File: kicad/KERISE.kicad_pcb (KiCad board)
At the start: 2 copper layers, 46.5 x 50 mm, 145 parts, among them J1 COM, P1 ANT, P10 Partition, P11 PR_Host, P12 PR_Slave, P13 Partition, P14 Partition, P15 Partition, P16 Partition, P17 Fan, P18 ENC_Host, P19 ENC_Slave, P2 Motor_L, P20 ToF_Host, P21 ToF_Slave, P22 ENC_Host, P23 ENC_Slave, P24 PR_Host, P25 PR_Slave, P26 Partition, P27 Partition, P28 Partition, P29 Partition, P3 Motor_R, P30 PR_Host, P31 PR_Slave, P32 Partition, P33 Partition, P34 Partition, P35 Partition, P4 Battery, P5 PR_Host, P6 PR_Slave, P7 Partition, P8 Partition, P9 Partition, Q1 DMN3065LW-7, Q2 DMN3065LW-7, Q3 NX3020NAKW, Q4 DMN3065LW-7, Q5 DMN3065LW-7, Q6 DMN3065LW-7, SW1 SW_Push, SW2 SW_Push, U1 FLASH, U10 AS5048A, U11 ICM-20602, U12 AD8601, U13 AD8601, U2 ESP32, U3 XTAL, U4 DRV8835, U5 LXDC2URxx, U6 AD8601, U7 AD8601, U8 AS5048A, U9 VL53L0X

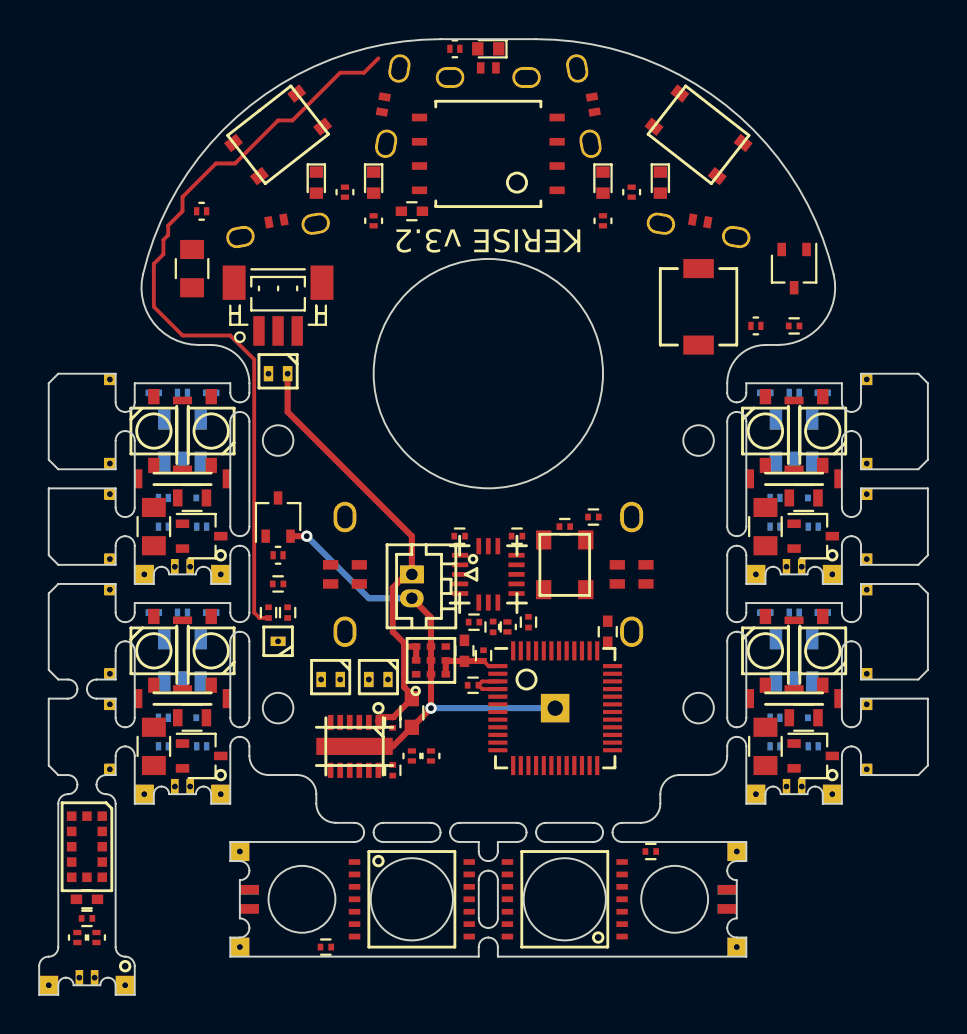
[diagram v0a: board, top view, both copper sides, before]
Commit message: 配線完了
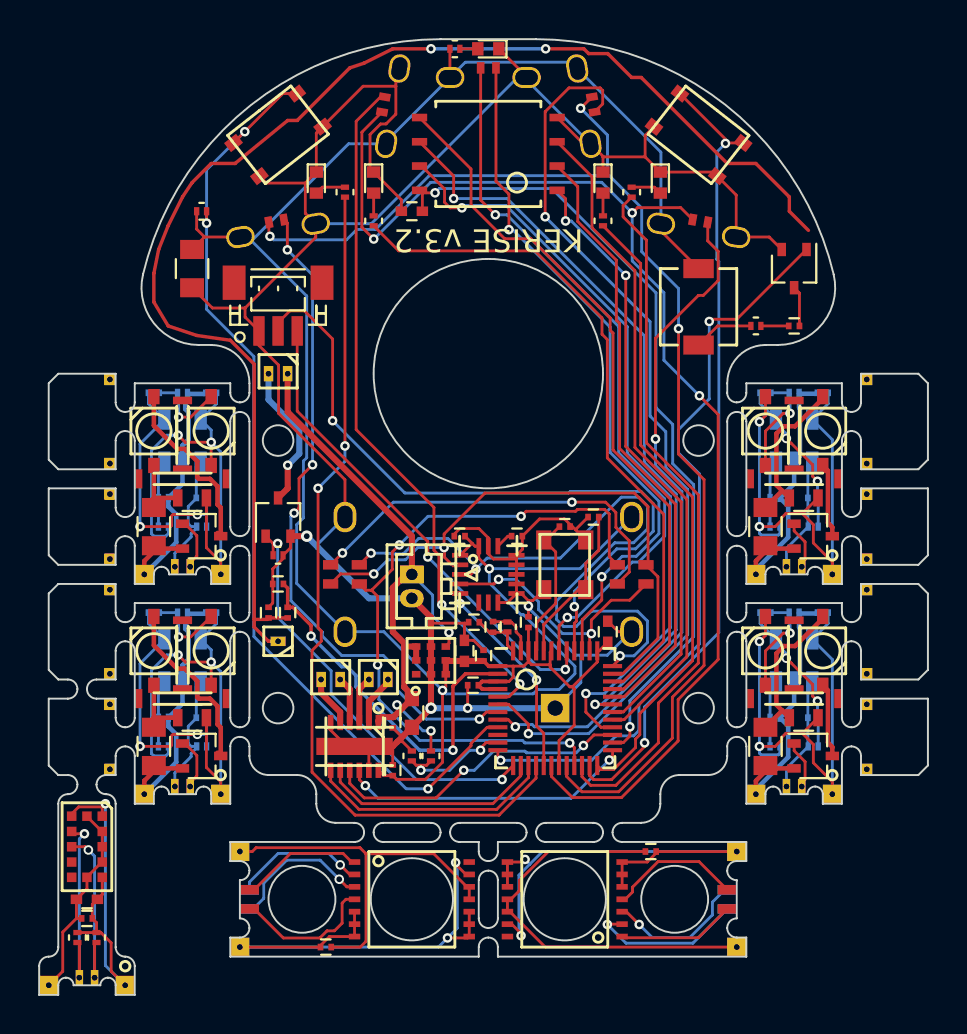
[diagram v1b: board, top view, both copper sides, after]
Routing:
- net GND: track 25.2 -> 155.0 mm, vias 2 -> 4
- net +3V3: track 6.01 -> 127.3 mm, vias 0 -> 2
- net PR-LED-SL: track 0.00 -> 65.5 mm, vias 0 -> 3
- net PR-LED-SR: track 0.00 -> 64.7 mm, vias 0 -> 3
- net Net-(R2-Pad1): track 0.00 -> 50.7 mm, vias 0 -> 3
- net PR-RCV-SR: track 0.00 -> 48.3 mm, vias 0 -> 2
- net LED_4: track 0.00 -> 45.1 mm, vias 0 -> 2
- net VDD_SDIO: track 0.00 -> 42.2 mm, vias 0 -> 2
- net BUTTON: track 0.00 -> 42.1 mm, vias 0 -> 2
- net SHD/SD2: track 0.00 -> 40.1 mm, vias 0 -> 2
- net SCK/CLK: track 0.00 -> 39.5 mm, vias 0 -> 2
- net SPEAKER: track 0.00 -> 39.0 mm, vias 0 -> 2
- net SDI/SD1: track 0.00 -> 37.7 mm
- net I2C-SDA: track 0.00 -> 37.6 mm, vias 0 -> 2
- net UART-RX: track 0.00 -> 37.1 mm, vias 0 -> 2
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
